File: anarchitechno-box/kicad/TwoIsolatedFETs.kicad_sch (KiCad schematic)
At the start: 2 parts, among them U1 TC4426xOA, U2 ADuM1200AR

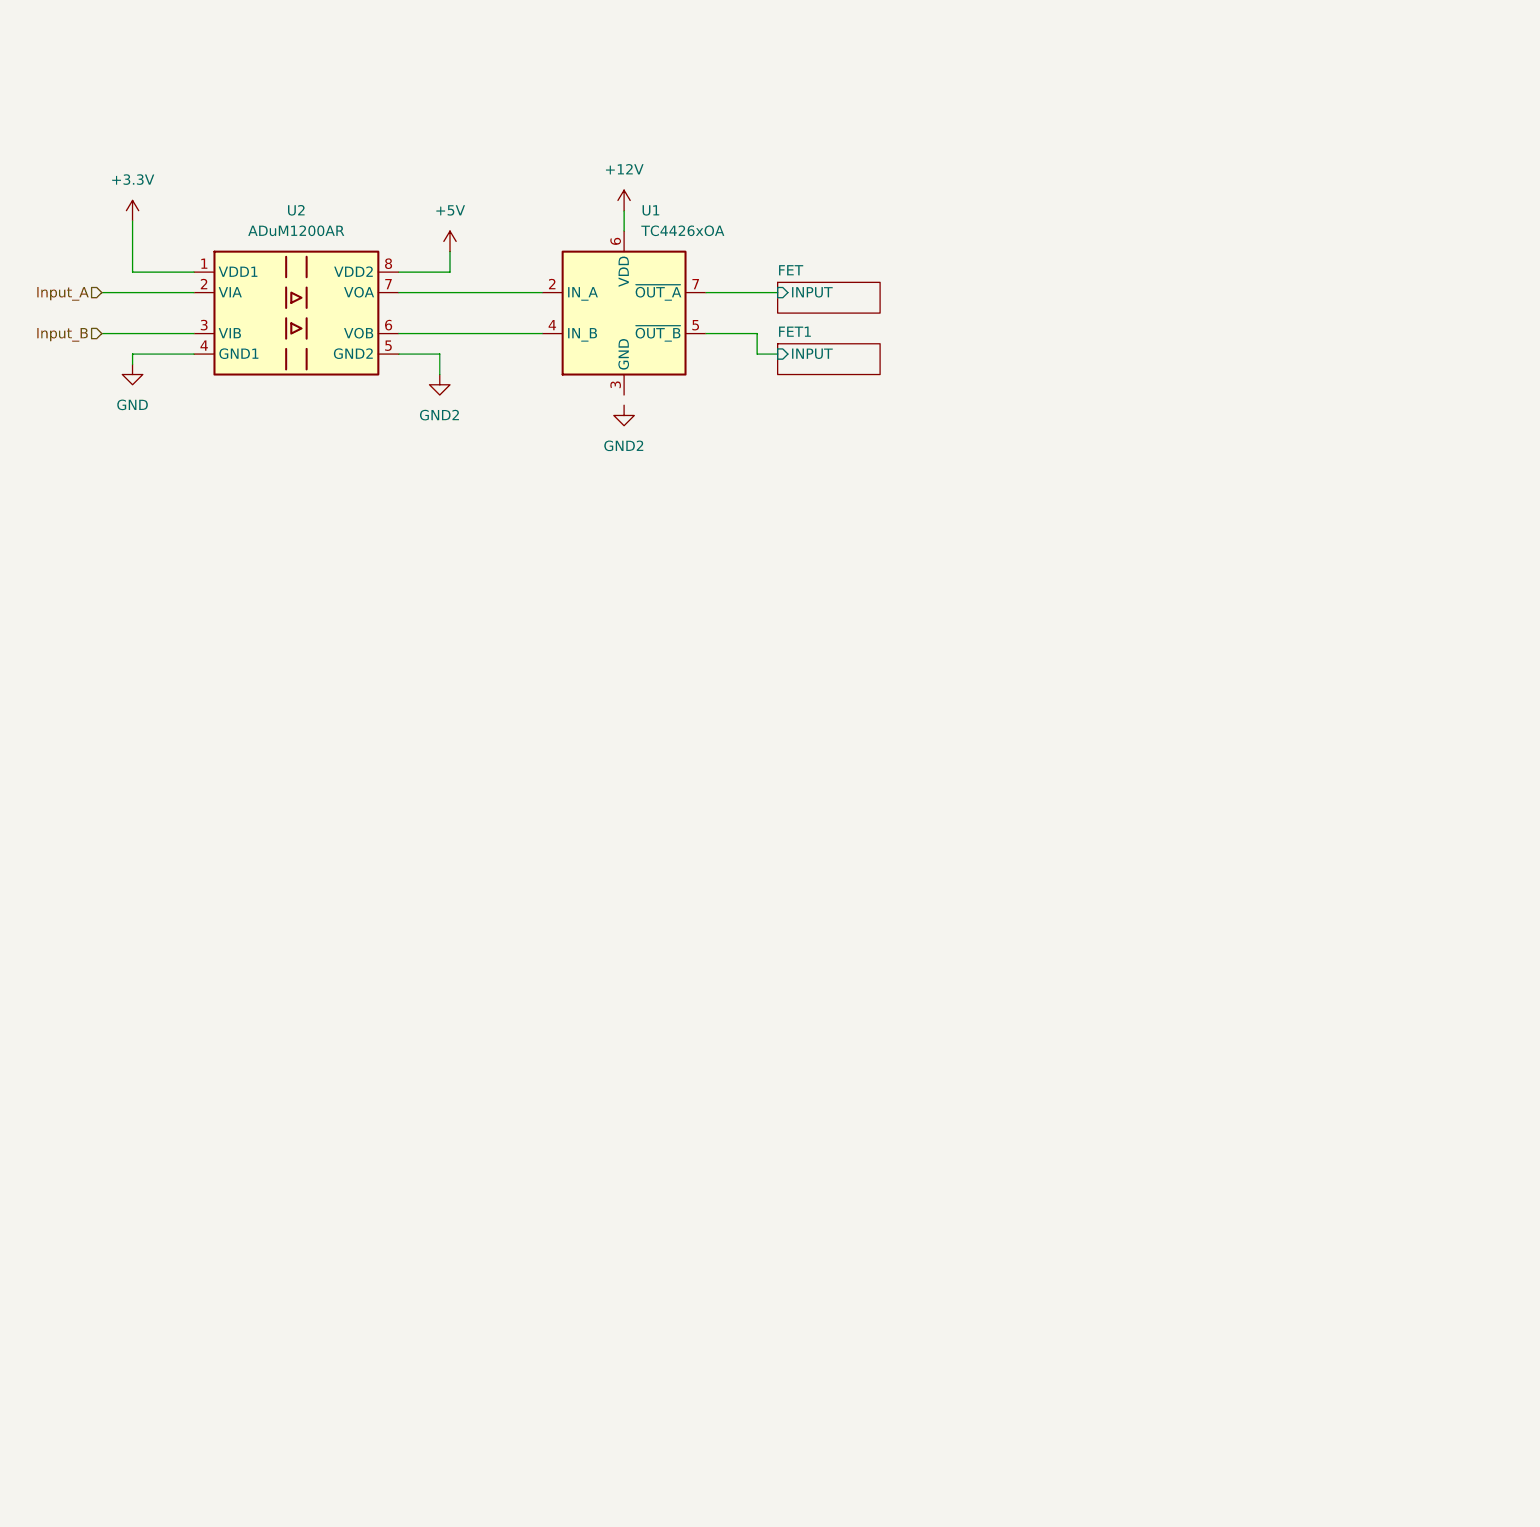
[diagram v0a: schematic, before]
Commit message: Large intermediate schematic push. Remaining todos are on frontpage.
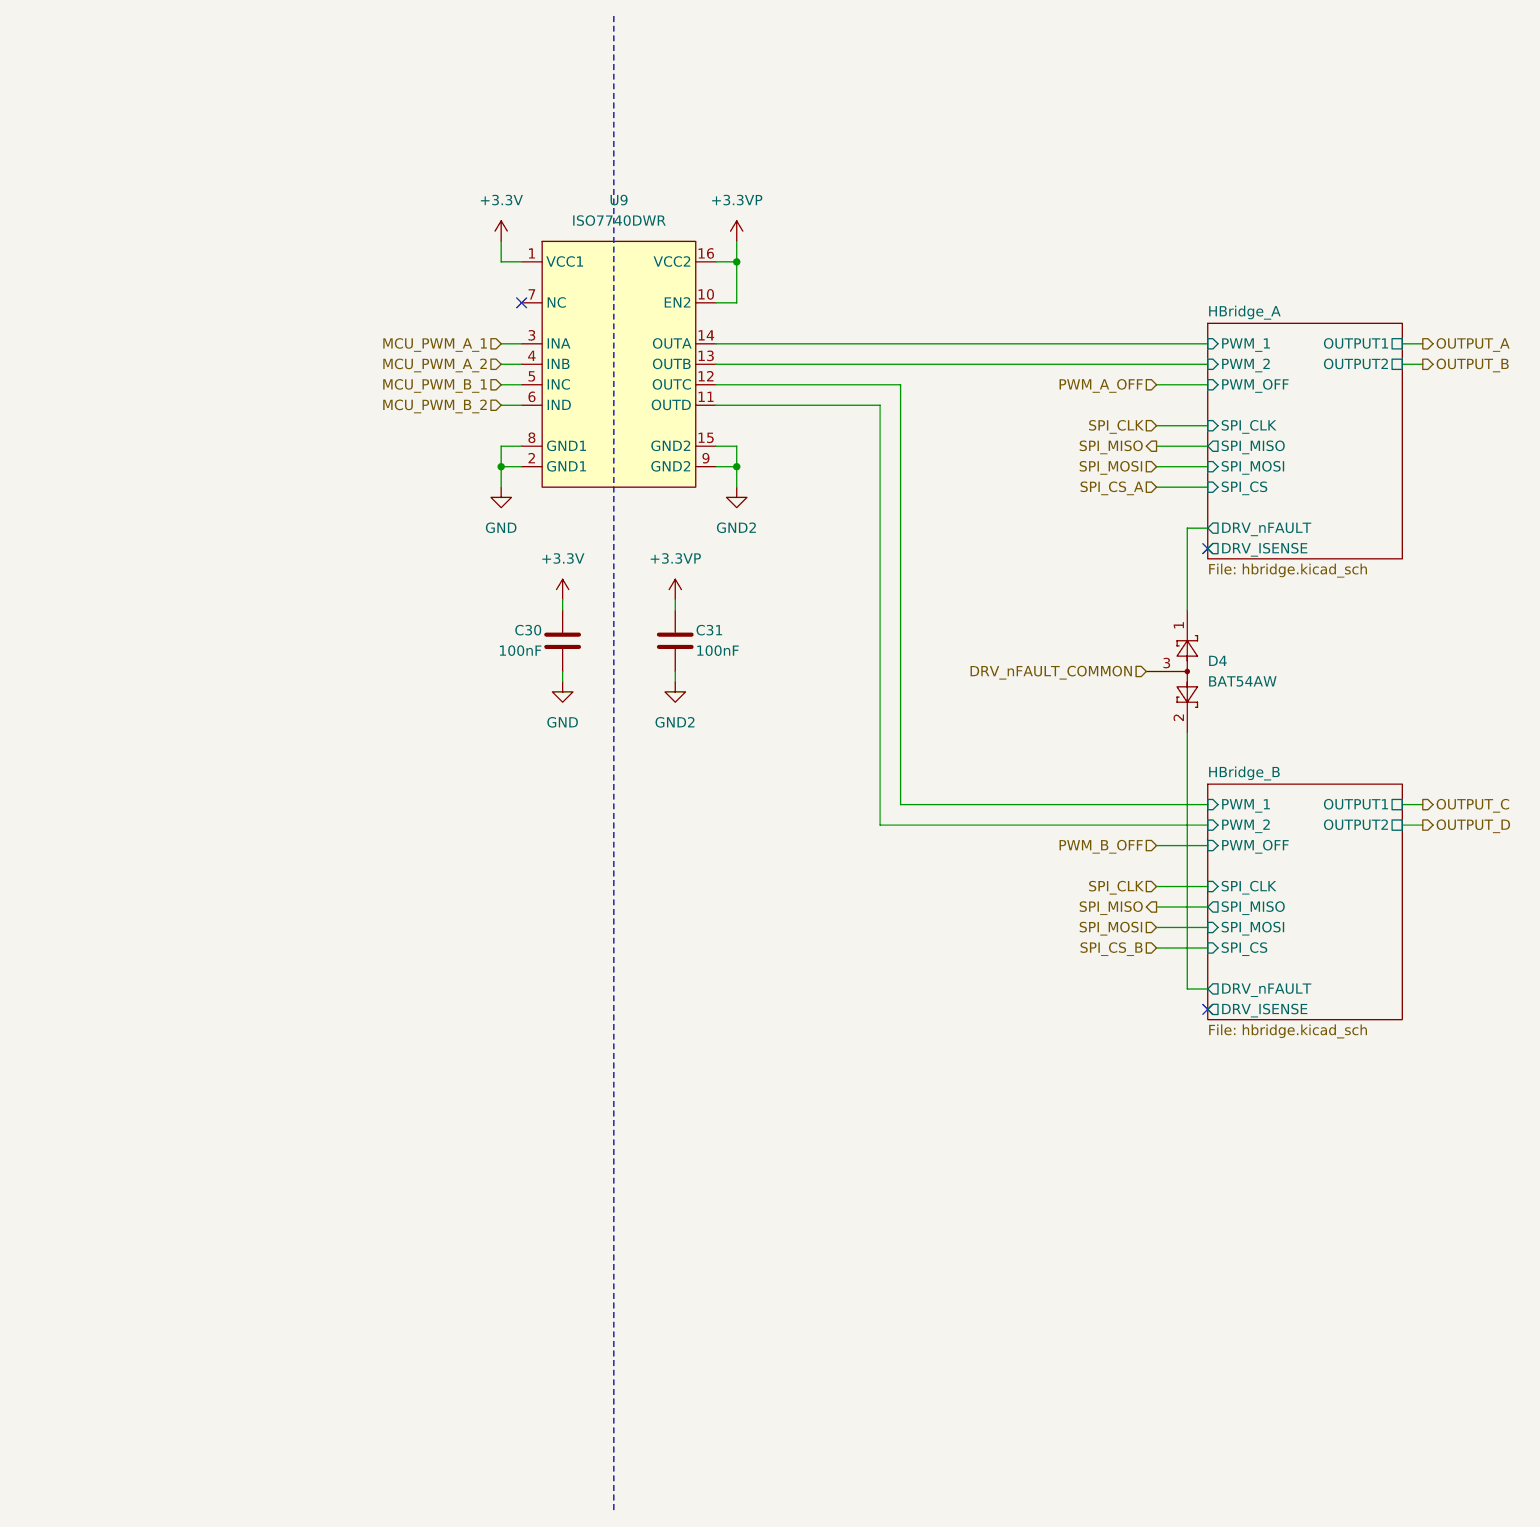
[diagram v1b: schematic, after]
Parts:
- removed U1: TC4426xOA, Package_SO:SOIC-8_3.9x4.9mm_P1.27mm, symbol Driver_FET:TC4426xOA
- removed U2: ADuM1200AR, Package_SO:SOIC-8_3.9x4.9mm_P1.27mm, symbol Isolator:ADuM1200AR
- added C30, C31: 100nF, Capacitor_SMD:C_0402_1005Metric, symbol Device:C
- added D4: BAT54AW, Package_TO_SOT_SMD:SOT-323_SC-70, symbol Diode:BAT54AW
- added U9: ISO7740DWR, Package_SO:SOIC-16W_7.5x10.3mm_P1.27mm, symbol parts:ISO7740
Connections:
- net +3.3V: now also C30.1, U9.1 (VCC1)
- net GND: now also C30.2, U9.2 (GND1), U9.8 (GND1)
- net GND2: now also C31.2, U9.15 (GND2), U9.9 (GND2)
- new net +3.3VP: C31.1, U9.10 (EN2), U9.16 (VCC2)
- new net DRV_nFAULT_COMMON: D4.3
- new net HBridge_A/DRV_nFAULT: D4.1
- new net HBridge_A/PWM_1: U9.14 (OUTA)
- new net HBridge_A/PWM_2: U9.13 (OUTB)
- new net HBridge_B/DRV_nFAULT: D4.2
- new net HBridge_B/PWM_1: U9.12 (OUTC)
- new net HBridge_B/PWM_2: U9.11 (OUTD)
- new net MCU_PWM_A_1: U9.3 (INA)
- new net MCU_PWM_A_2: U9.4 (INB)
- new net MCU_PWM_B_1: U9.5 (INC)
- new net MCU_PWM_B_2: U9.6 (IND)
- no-connect marks 0 -> 3
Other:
- removed sheet FET
- removed sheet FET1
- added sheet HBridge_A (hbridge.kicad_sch)
- added sheet HBridge_B (hbridge.kicad_sch)
